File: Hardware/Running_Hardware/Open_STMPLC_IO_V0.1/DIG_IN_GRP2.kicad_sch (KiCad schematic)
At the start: 68 parts, among them J3 Screw_Terminal_01x04, J8 Screw_Terminal_01x04, U12 6N137, U20 6N137, U21 6N137, U22 6N137, U23 6N137, U24 6N137

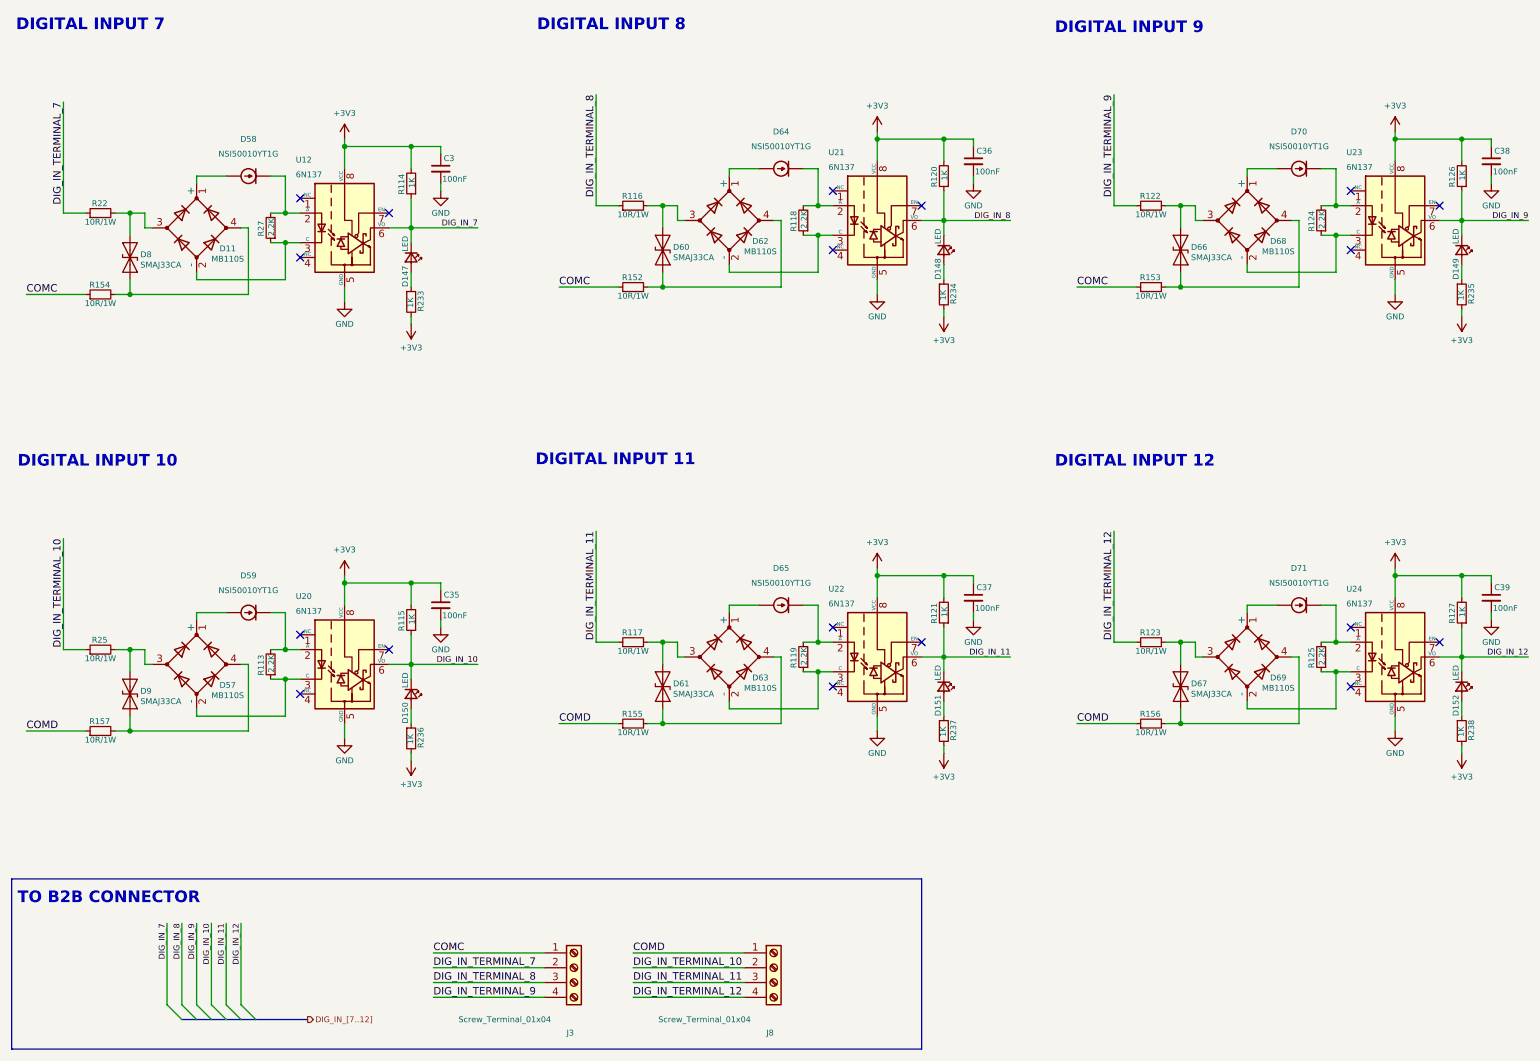
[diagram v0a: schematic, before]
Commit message: Main PCB changes
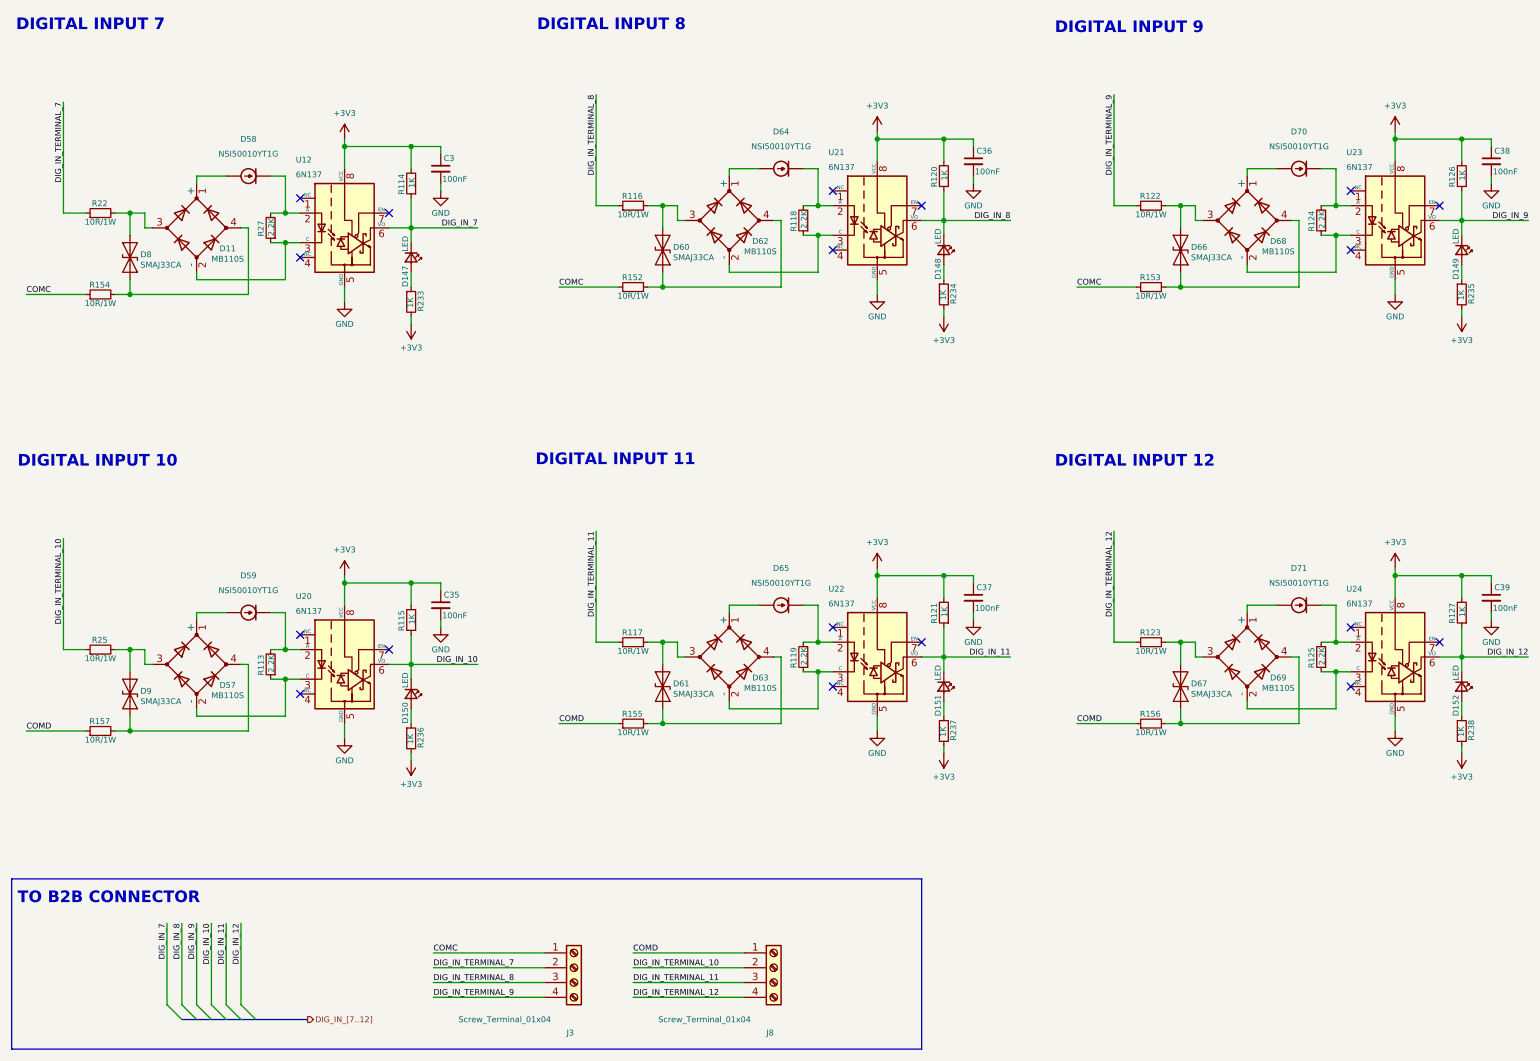
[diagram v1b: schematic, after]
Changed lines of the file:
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@@
 		(effects
 			(font
-				(size 1.27 1.27)
+				(size 1 1)
 			)
 			(justify left bottom)
@@
 		(effects
 			(font
-				(size 1.27 1.27)
+				(size 1 1)
 			)
 			(justify right bottom)
@@
 		(effects
 			(font
-				(size 1.27 1.27)
+				(size 1 1)
 			)
 			(justify left bottom)
@@
 		(effects
 			(font
-				(size 1.27 1.27)
+				(size 1 1)
 			)
 			(justify right bottom)
@@
 		(effects
 			(font
-				(size 1.27 1.27)
+				(size 1 1)
 			)
 			(justify left bottom)
@@
 		(effects
 			(font
-				(size 1.27 1.27)
+				(size 1 1)
 			)
 			(justify left bottom)
@@
 		(effects
 			(font
-				(size 1.27 1.27)
+				(size 1 1)
 			)
 			(justify left bottom)
@@
 		(effects
 			(font
-				(size 1.27 1.27)
+				(size 1 1)
 			)
 			(justify left bottom)
@@
 		(effects
 			(font
-				(size 1.27 1.27)
+				(size 1 1)
 			)
 			(justify left bottom)
@@
 		(effects
 			(font
-				(size 1.27 1.27)
+				(size 1 1)
 			)
 			(justify right bottom)
@@
 		(effects
 			(font
-				(size 1.27 1.27)
+				(size 1 1)
 			)
 			(justify left bottom)
@@
 		(effects
 			(font
-				(size 1.27 1.27)
+				(size 1 1)
 			)
 			(justify left bottom)
@@
 		(effects
 			(font
-				(size 1.27 1.27)
+				(size 1 1)
 			)
 			(justify left bottom)
@@
 		(effects
 			(font
-				(size 1.27 1.27)
+				(size 1 1)
 			)
 			(justify right bottom)
@@
 		(effects
 			(font
-				(size 1.27 1.27)
+				(size 1 1)
 			)
 			(justify left bottom)
@@
 		(effects
 			(font
-				(size 1.27 1.27)
+				(size 1 1)
 			)
 			(justify right bottom)
@@
 		(effects
 			(font
-				(size 1.27 1.27)
+				(size 1 1)
 			)
 			(justify left bottom)
@@
 		(effects
 			(font
-				(size 1.27 1.27)
+				(size 1 1)
 			)
 			(justify left bottom)
@@
 		(effects
 			(font
-				(size 1.27 1.27)
+				(size 1 1)
 			)
 			(justify left bottom)
@@
 		(effects
 			(font
-				(size 1.27 1.27)
-			)
-			(justify right bottom)
+				(size 1 1)
+			)
+			(justify right bottom)
